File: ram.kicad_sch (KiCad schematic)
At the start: 2 parts, among them U5 MT41K256M16TW

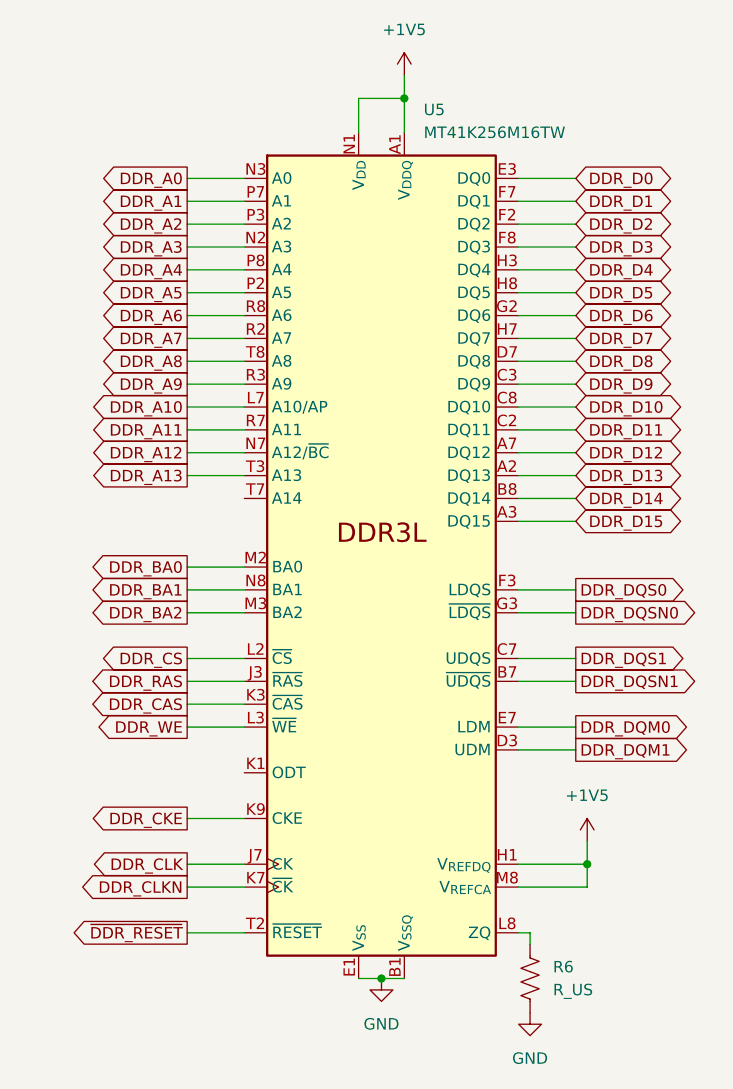
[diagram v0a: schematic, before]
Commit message: morning
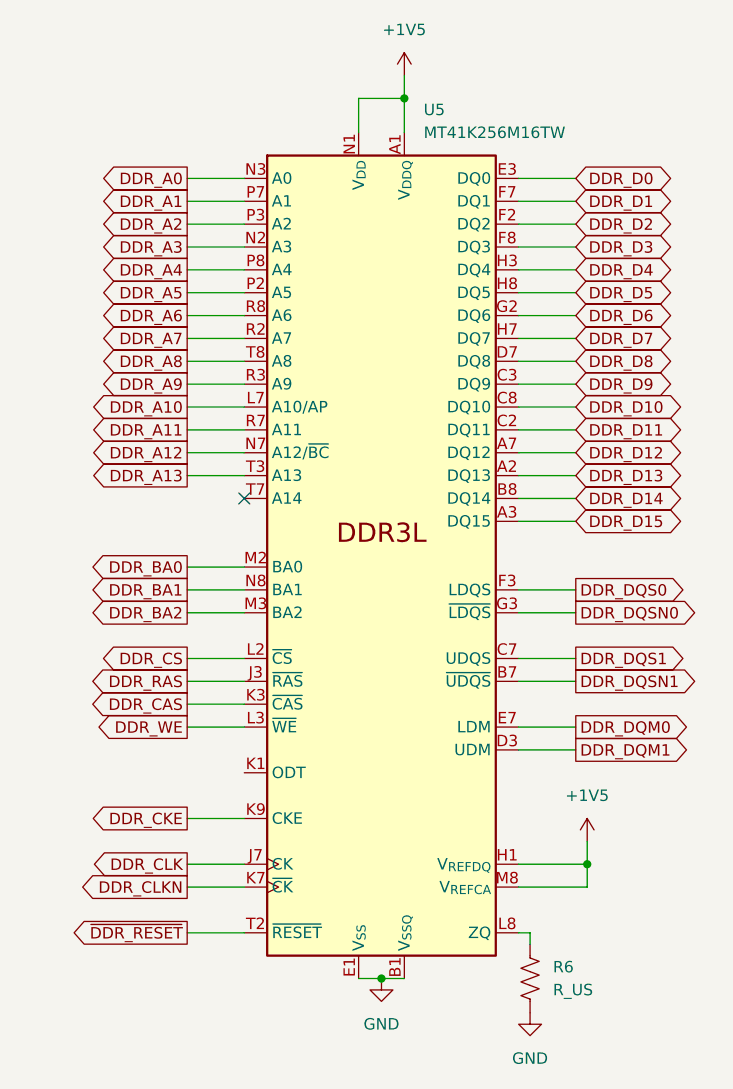
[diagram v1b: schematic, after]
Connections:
- no-connect marks 0 -> 1
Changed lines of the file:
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@@
 		(color 0 0 0 0)
+	)
+	(no_connect
+		(at 138.43 91.44)
 	)
 	(wire

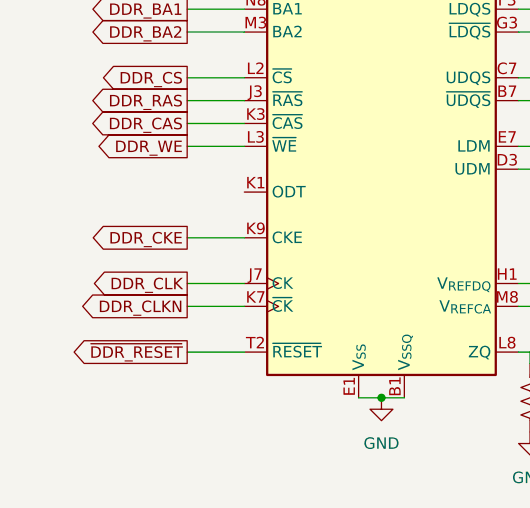
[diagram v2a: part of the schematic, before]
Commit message: after rough draft submission
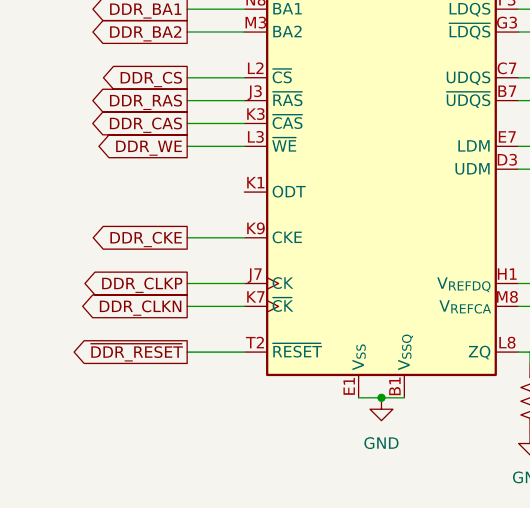
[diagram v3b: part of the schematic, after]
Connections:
- net DDR_CLK renamed DDR_CLKP
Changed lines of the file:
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@@
 		)
 	)
-	(global_label "DDR_CLK"
+	(global_label "DDR_CLKP"
 		(shape output)
 		(at 132.08 132.08 180)
